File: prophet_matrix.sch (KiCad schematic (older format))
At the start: 132 parts

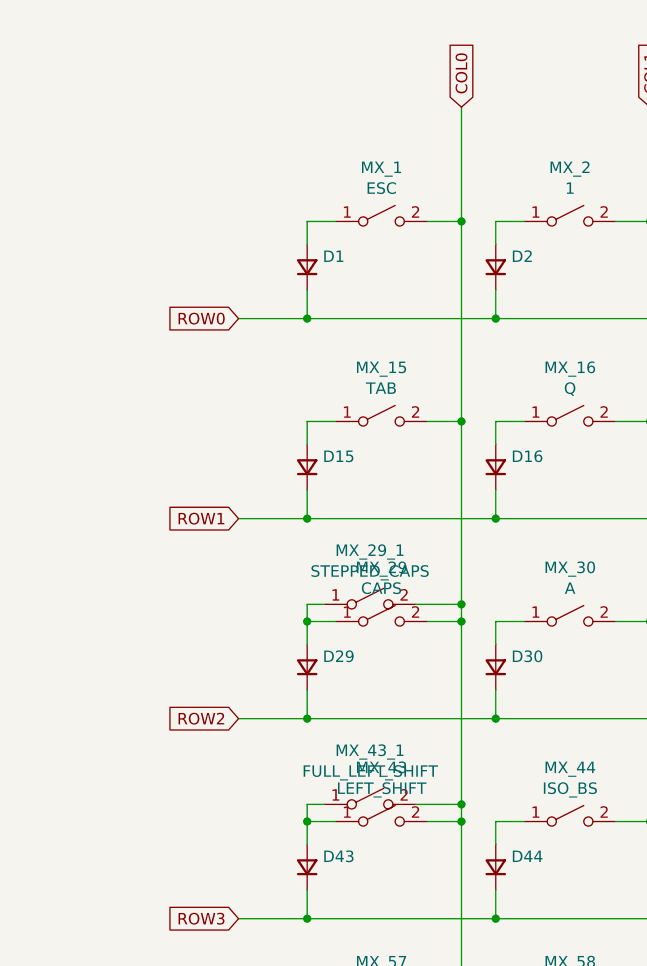
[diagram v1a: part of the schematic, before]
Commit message: update to latest rev
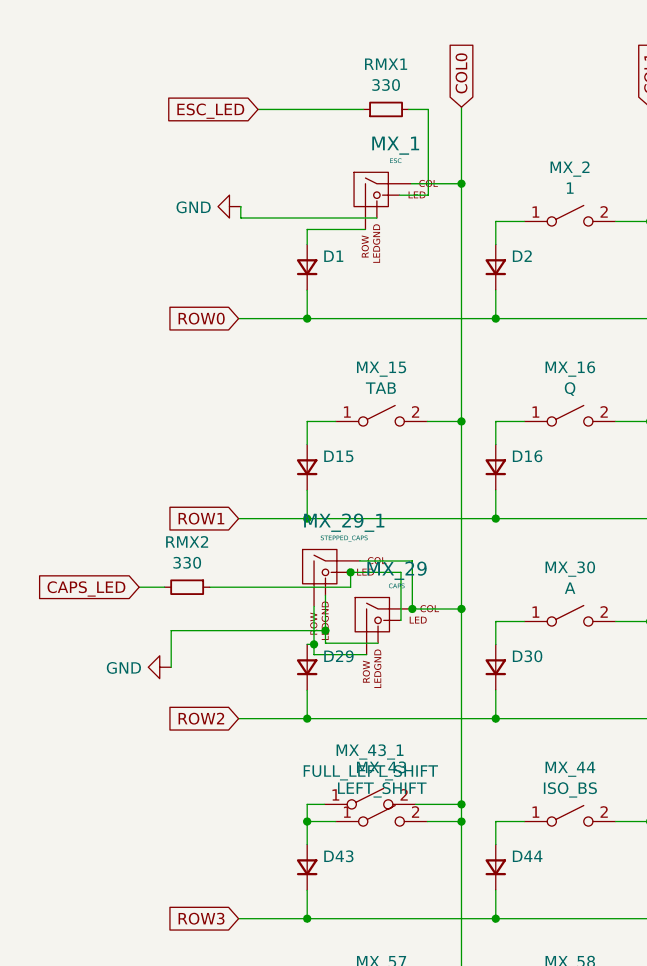
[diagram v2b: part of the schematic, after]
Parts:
- removed MX_1: ESC, MX_Alps_Hybrid:MXOnly-1U-NoLED, symbol Switch:SW_SPST
- removed MX_29: CAPS, MX_Alps_Hybrid:MXOnly-1.75U-NoLED, symbol Switch:SW_SPST
- removed MX_29_1: STEPPED_CAPS, MX_Alps_Hybrid:MXOnly-1.25U-NoLED, symbol Switch:SW_SPST
- added MX_1: ESC, MX_Only:MXOnly-1U, symbol MX_Alps_Hybrid:MX-LED
- added MX_29: CAPS, MX_Only:MXOnly-1.75U, symbol MX_Alps_Hybrid:MX-LED
- added MX_29_1: STEPPED_CAPS, MX_Only:MXOnly-1.25U, symbol MX_Alps_Hybrid:MX-LED
- added RMX1, RMX2: 330, Resistor_SMD:R_0805_2012Metric, symbol Device:R_Small
- D1, D10, D11, D12, D13, D14, D15, D16, D17, D18, D19, D2, D20, D21, D22, D23, D24, D25, D26, D27, D28, D29, D3, D30, D31, D32, D33, D34, D35, D36, D37, D38, D39, D4, D40, D42, D43, D44, D45, D46, D47, D48, D49, D5, D50, D51, D52, D53, D54, D55, D56, D57, D58, D59, D6, D60, D61, D62, D63, D64, D7, D8, D9: footprint Diode_SMD:D_0805_2012Metric_Pad1.15x1.40mm_HandSolder -> Diode_SMD:D_0805_2012Metric
- MX_10, MX_11, MX_12, MX_13, MX_14_1, MX_16, MX_17, MX_18, MX_19, MX_2, MX_20, MX_21, MX_22, MX_23, MX_24, MX_25, MX_26, MX_27, MX_3, MX_30, MX_31, MX_32, MX_33, MX_34, MX_35, MX_36, MX_37, MX_38, MX_39, MX_4, MX_40, MX_44, MX_45, MX_46, MX_47, MX_48, MX_49, MX_5, MX_50, MX_51, MX_52, MX_53, MX_54, MX_56, MX_58, MX_6, MX_62, MX_64, MX_7, MX_8, MX_9: footprint MX_Alps_Hybrid:MXOnly-1U-NoLED -> MX_Only:MXOnly-1U-NoLED
- MX_14: footprint MX_Alps_Hybrid:MXOnly-2U-NoLED -> MX_Only:MXOnly-2U-NoLED
- MX_15, MX_28, MX_57, MX_59, MX_61, MX_63: footprint MX_Alps_Hybrid:MXOnly-1.5U-NoLED -> MX_Only:MXOnly-1.5U-NoLED
- MX_42, MX_43_1: footprint MX_Alps_Hybrid:MXOnly-2.25U-NoLED -> MX_Only:MXOnly-2.25U-NoLED
- MX_43: footprint MX_Alps_Hybrid:MXOnly-1.25U-NoLED -> MX_Only:MXOnly-1.25U-NoLED
- MX_55: footprint MX_Alps_Hybrid:MXOnly-1.75U-NoLED -> MX_Only:MXOnly-1.75U-NoLED
- MX_55_1: footprint MX_Alps_Hybrid:MXOnly-2.75U-NoLED -> MX_Only:MXOnly-2.75U-NoLED
- MX_60: footprint MX_Alps_Hybrid:MXOnly-7U-ReversedStabilizers-NoLED -> MX_Only:MXOnly-7U-ReversedStabilizers-NoLED
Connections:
- net COL0: now also MX_1.1 (COL), MX_29.1 (COL), MX_29_1.1 (COL)
- net at D1.2 (A): now also MX_1.2 (ROW)
- net at D29.2 (A): now also MX_29.2 (ROW), MX_29_1.2 (ROW)
- new net: MX_1.3 (LED), RMX1.2
- new net: MX_29.3 (LED), MX_29_1.3 (LED), RMX2.1
- new net CAPS_LED: RMX2.2
- new net ESC_LED: RMX1.1
- new net GND: MX_1.4 (LEDGND), MX_29.4 (LEDGND), MX_29_1.4 (LEDGND)
